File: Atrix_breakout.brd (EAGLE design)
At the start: 8.1 x 17.4 mm, 9 parts

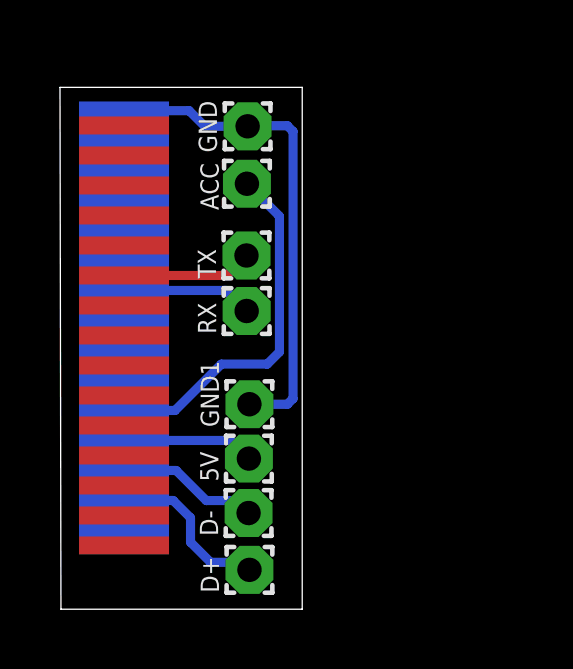
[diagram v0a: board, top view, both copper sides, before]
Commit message: Push to OpenJB
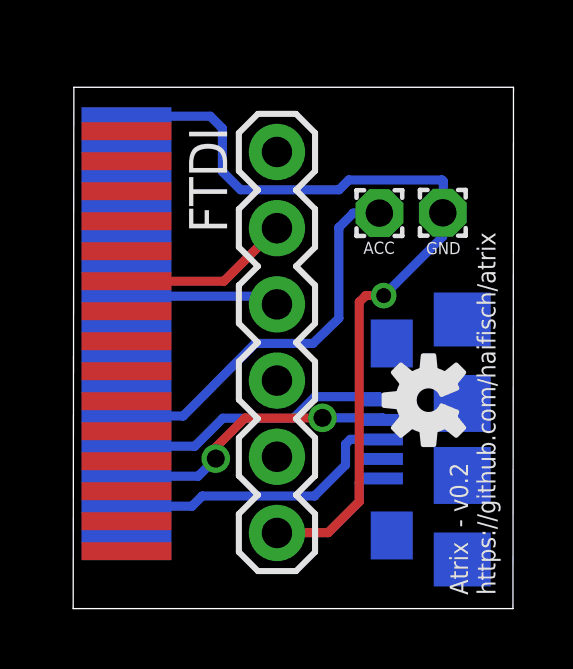
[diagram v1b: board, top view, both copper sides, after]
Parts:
- removed 5V, D+, D-, GND1, RX, TX: (no value), wirepad:1,6/0,8
- added JP1: FTDI, SparkFun-Connectors:FTDI_BASIC
- added U$2: (no value), SparkFun-Aesthetics:OSHW-LOGO-S
- added X1: USB-MICROB, Pinoccio:USB-MICROB
- ACC, GND: device wirepad:1,6/0,8 -> wirepad:1,6/0,9
- moved GND 7.12 mm to (10.7, 16.8), turned to 180 degrees
- moved ACC 4.52 mm to (8.61, 16.8), turned to 180 degrees
- moved U$1 0.21 mm to (0.18, 12.5)
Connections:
- removed net N$3: D-.1, U$1.25
- removed net N$4: D+.1, U$1.27
- removed net N$6: RX.1, U$1.13
- removed net N$7: TX.1, U$1.12
- removed net N$8: 5V.1, U$1.23
- new net 5V: U$1.23, X1.VBUS
- new net D+: U$1.27, X1.D+
- new net D-: U$1.25, X1.D-
- new net RX: JP1.TXO, U$1.13
- new net TX: JP1.RXI, U$1.12
- net GND: now also JP1.GND, X1.GND; no longer GND1.1
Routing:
- net GND: track 16.4 -> 32.6 mm, vias 0 -> 1
- net D+: track 0.00 -> 9.87 mm
- net D-: track 0.00 -> 9.64 mm, vias 0 -> 2
- net 5V: track 0.00 -> 9.28 mm
- net TX: track 0.00 -> 5.75 mm
- net N$4: track 5.62 -> 0.00 mm
- net RX: track 0.00 -> 5.13 mm
- net N$3: track 4.74 -> 0.00 mm
- net N$8: track 4.41 -> 0.00 mm
- net N$6: track 4.37 -> 0.00 mm
- net N$7: track 4.36 -> 0.00 mm
- net N$1: track 12.0 -> 13.0 mm
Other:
- board size 8.1 x 17.4 mm -> 14.7 x 17.4 mm
- board text added: "Atrix - v0.2 https://github.com/haifisch/atrix"
